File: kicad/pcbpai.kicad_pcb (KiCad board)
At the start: 2 copper layers, 78.7 x 98 mm, 20 parts, among them J1 Fuse, J2 Conn_01x04_Pin, J3 Input 24 V, J4 Boton Encendido, J5 Parada de Emergencia, J6 Conn_01x06_Pin, J7 Raspberry GPIO, J8 Conn_01x09_Pin, J9 Conn_01x02_Socket, M1 MountingHole_2.5mm_Pad, M2 MountingHole_2.5mm_Pad, M3 MountingHole_2.5mm_Pad, M4 MountingHole_2.5mm_Pad, SW1 SW_Push_DPDT, U6 ATtiny85-20P

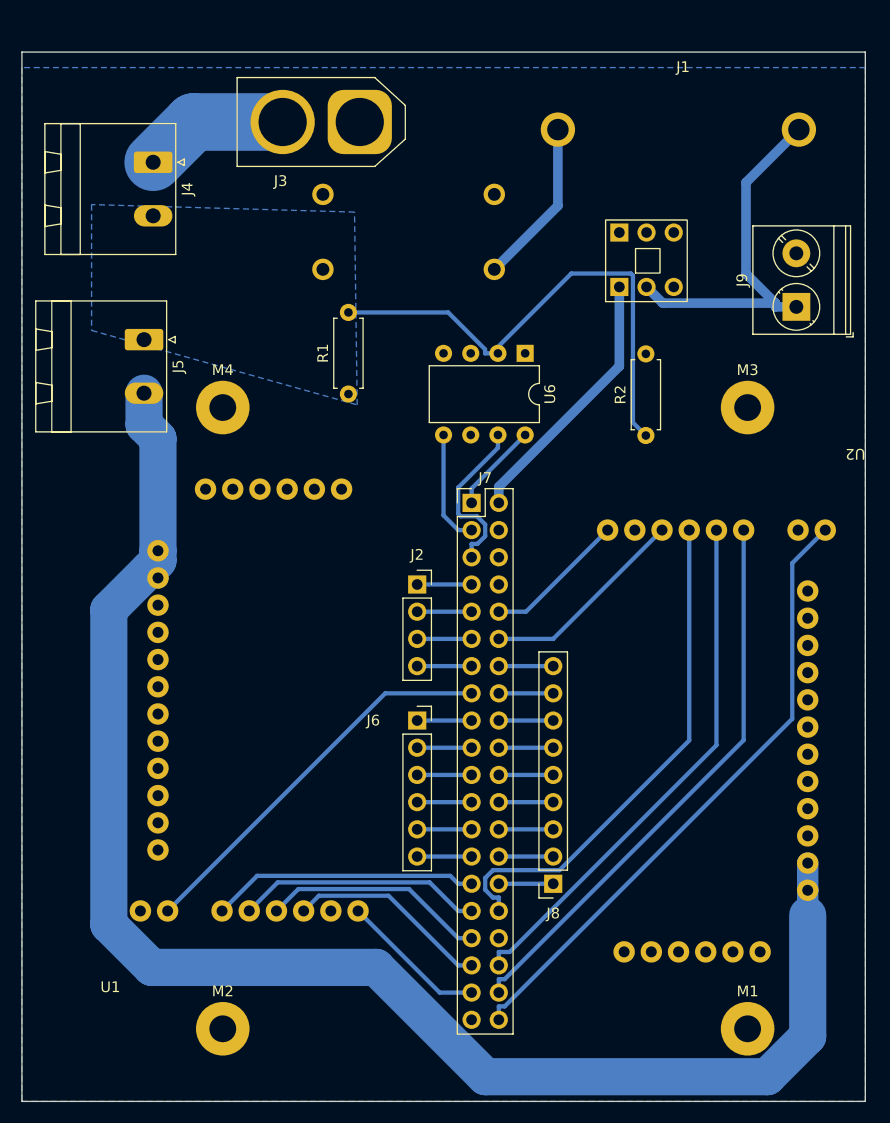
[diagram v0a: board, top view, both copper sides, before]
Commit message: finish pcb
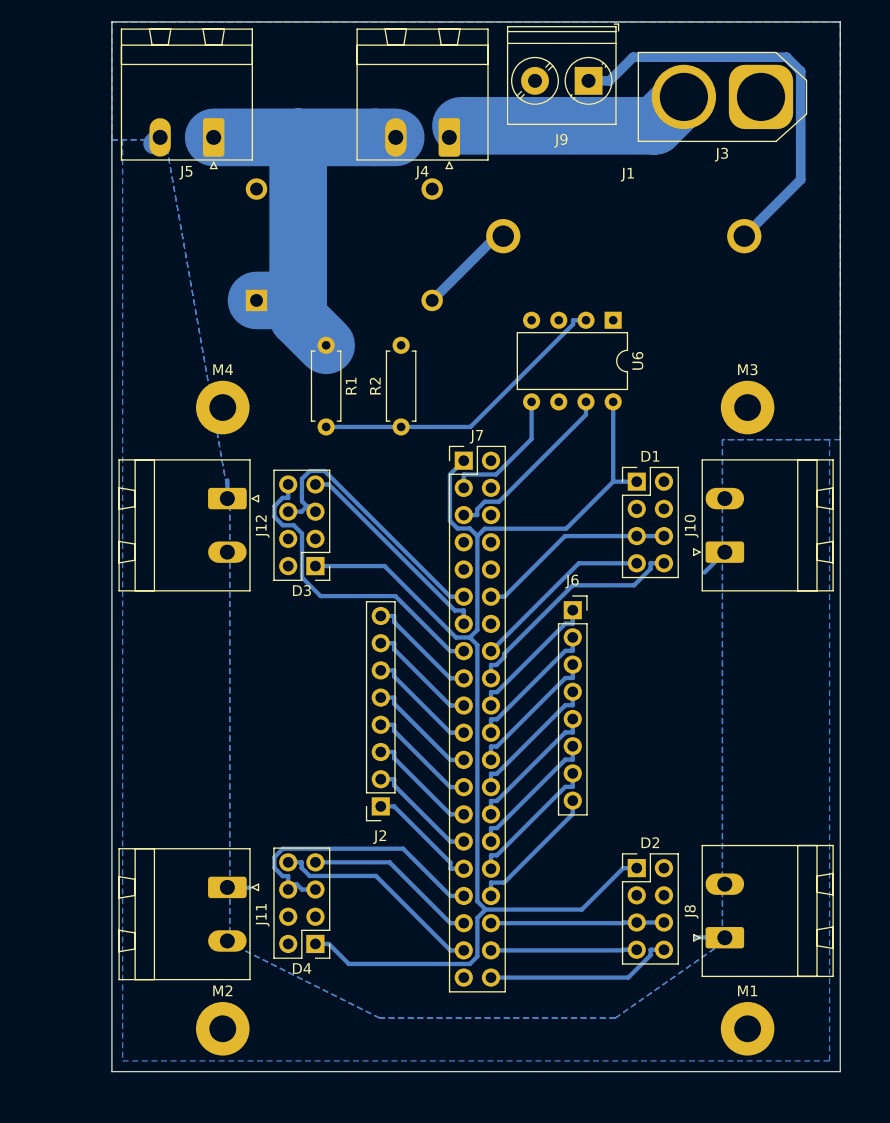
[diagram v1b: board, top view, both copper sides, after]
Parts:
- removed SW1: SW_Push_DPDT, PAI:switch
- removed U1, U2: ~, PAI:Pololu MAX 14870 Dual Shield Arduino
- added D1: ~, Connector_PinHeader_2.54mm:PinHeader_2x04_P2.54mm_Vertical, F.Cu at (159.0, 86.9)
- added D2: ~, Connector_PinHeader_2.54mm:PinHeader_2x04_P2.54mm_Vertical, F.Cu at (159.0, 123.0)
- added D3: ~, Connector_PinHeader_2.54mm:PinHeader_2x04_P2.54mm_Vertical, F.Cu at (129.0, 94.8)
- added D4: ~, Connector_PinHeader_2.54mm:PinHeader_2x04_P2.54mm_Vertical, F.Cu at (129.0, 130.1)
- added J10: Conn_01x02_Socket, Connector_Phoenix_MSTB:PhoenixContact_MSTBA_2,5_2-G_1x02_P5.00mm_Horizontal, F.Cu at (167.2, 93.5)
- added J11: Conn_01x02_Socket, Connector_Phoenix_MSTB:PhoenixContact_MSTBA_2,5_2-G_1x02_P5.00mm_Horizontal, F.Cu at (120.8, 124.8)
- added J12: Conn_01x02_Socket, Connector_Phoenix_MSTB:PhoenixContact_MSTBA_2,5_2-G_1x02_P5.00mm_Horizontal, F.Cu at (120.8, 88.5)
- J2: value Conn_01x04_Pin -> Conn_01x08_Socket; footprint Connector_PinSocket_2.54mm:PinSocket_1x04_P2.54mm_Vertical -> Connector_PinSocket_2.54mm:PinSocket_1x08_P2.54mm_Vertical
- J6: value Conn_01x06_Pin -> Conn_01x08_Socket; footprint Connector_PinSocket_2.54mm:PinSocket_1x06_P2.54mm_Vertical -> Connector_PinSocket_2.54mm:PinSocket_1x08_P2.54mm_Vertical
- J8: value Conn_01x09_Pin -> Conn_01x02_Socket; footprint Connector_PinSocket_2.54mm:PinSocket_1x09_P2.54mm_Vertical -> Connector_Phoenix_MSTB:PhoenixContact_MSTBA_2,5_2-G_1x02_P5.00mm_Horizontal
- U4: footprint PAI:regulador -> PAI:regulator
- moved J3 37.5 mm to (170.6, 51.0)
- moved J9 28.7 mm to (154.5, 49.5), turned to 180 degrees
- moved J4 27.7 mm to (141.5, 54.8), turned to 180 degrees
- moved U4 23.3 mm to (123.5, 70.0), turned to 0 degrees
- moved R2 22.9 mm to (137.0, 81.8)
- moved J2 21.0 mm to (135.1, 117.2), turned to 180 degrees
- moved J5 20.0 mm to (119.5, 54.8), turned to 180 degrees
- moved J6 17.8 mm to (153.0, 98.9)
- moved J8 16.8 mm to (167.2, 129.5), turned to 90 degrees
- moved J1 11.2 mm to (146.5, 64.0)
- moved U6 8.78 mm to (156.8, 71.8)
- moved R1 5.00 mm to (130.0, 74.2), turned to -90 degrees
- moved J7 4.01 mm to (142.8, 85.0)
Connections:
- net Net-(J7-Pin_1) renamed +3.3V
- J5 pad 2: Net-(J5-Pin_2) -> Net-(J10-Pin_2)
- J7 pad 10: Net-(J7-Pin_10) -> unconnected-(J7-Pin_10-Pad10)
- J7 pad 11: Net-(J2-Pin_3) -> Net-(D3-EL)
- J7 pad 13: Net-(J2-Pin_4) -> Net-(D3-PWMR)
- J7 pad 14: Net-(J7-Pin_14) -> unconnected-(J7-Pin_14-Pad14)
- J7 pad 16: Net-(J7-Pin_16) -> Net-(D1-PWMR)
- J7 pad 17: Net-(J6-Pin_1) -> Net-(J2-Pin_8)
- J7 pad 18: Net-(J7-Pin_18) -> Net-(D1-PWML)
- J7 pad 19: Net-(J6-Pin_2) -> Net-(J2-Pin_7)
- J7 pad 2: Net-(J7-Pin_2) -> unconnected-(J7-Pin_2-Pad2)
- J7 pad 20: Net-(J7-Pin_20) -> Net-(J6-Pin_1)
- J7 pad 21: Net-(J6-Pin_3) -> Net-(J2-Pin_6)
- J7 pad 22: Net-(J7-Pin_22) -> Net-(J6-Pin_2)
- J7 pad 23: Net-(J6-Pin_4) -> Net-(J2-Pin_5)
- J7 pad 24: Net-(J7-Pin_24) -> Net-(J6-Pin_3)
- J7 pad 25: Net-(J6-Pin_5) -> Net-(J2-Pin_4)
- J7 pad 26: Net-(J7-Pin_26) -> Net-(J6-Pin_4)
- J7 pad 27: Net-(J6-Pin_6) -> Net-(J2-Pin_3)
- J7 pad 28: Net-(J7-Pin_28) -> Net-(J6-Pin_5)
- J7 pad 29: Net-(J7-Pin_29) -> Net-(J2-Pin_2)
- J7 pad 30: Net-(J7-Pin_30) -> Net-(J6-Pin_6)
- J7 pad 31: Net-(J7-Pin_31) -> Net-(J2-Pin_1)
- J7 pad 32: Net-(J7-Pin_32) -> Net-(J6-Pin_7)
- J7 pad 34: unconnected-(J7-Pin_34-Pad34) -> Net-(J6-Pin_8)
- J7 pad 39: unconnected-(J7-Pin_39-Pad39) -> GND
- J7 pad 7: Net-(J2-Pin_1) -> unconnected-(J7-Pin_7-Pad7)
- J7 pad 9: Net-(J2-Pin_2) -> unconnected-(J7-Pin_9-Pad9)
- J8 pad 1: Net-(J7-Pin_30) -> GND
- J8 pad 2: Net-(J7-Pin_28) -> Net-(J10-Pin_2)
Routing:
- net Net-(J5-Pin_2): track 142.1 -> 0.00 mm
- net +3.3V: track 8.41 -> 123.3 mm
- net Net-(J7-Pin_32): track 47.9 -> 0.00 mm
- net Net-(J4-Pin_2): track 0.00 -> 41.4 mm
- net Net-(D2-PWML): track 58.7 -> 17.5 mm
- net Net-(D2-PWMR): track 53.0 -> 13.6 mm
- net Net-(D2-EL): track 49.6 -> 16.2 mm
- net Net-(D3-EL): track 0.00 -> 26.3 mm
- net Net-(J7-Pin_29): track 25.0 -> 0.00 mm
- net Net-(J7-Pin_2): track 24.8 -> 0.00 mm
- net Net-(J7-Pin_31): track 23.0 -> 0.00 mm
- net Net-(D1-PWML): track 0.00 -> 21.8 mm
- net Net-(D3-PWMR): track 0.00 -> 20.0 mm
- net Net-(U6-XTAL1/PB3): track 47.6 -> 28.6 mm
- net Net-(D1-PWMR): track 0.00 -> 17.0 mm
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- added copper zone on B.Cu, net Net-(J10-Pin_2)
- removed copper zone on B.Cu, net Net-(J4-Pin_2)
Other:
- board size 78.7 x 98 mm -> 68 x 98 mm
